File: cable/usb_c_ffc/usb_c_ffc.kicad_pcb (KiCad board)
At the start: 2 copper layers, 46.5 x 39.1 mm, 7 parts, among them J1 Conn_01x15_Socket, J2 Conn_01x15_Socket, J3 Conn_01x15_Socket, J4 Conn_01x15_Socket, J5 Conn_01x15_Socket, P1 TC-003LS, P2 TC-003LS

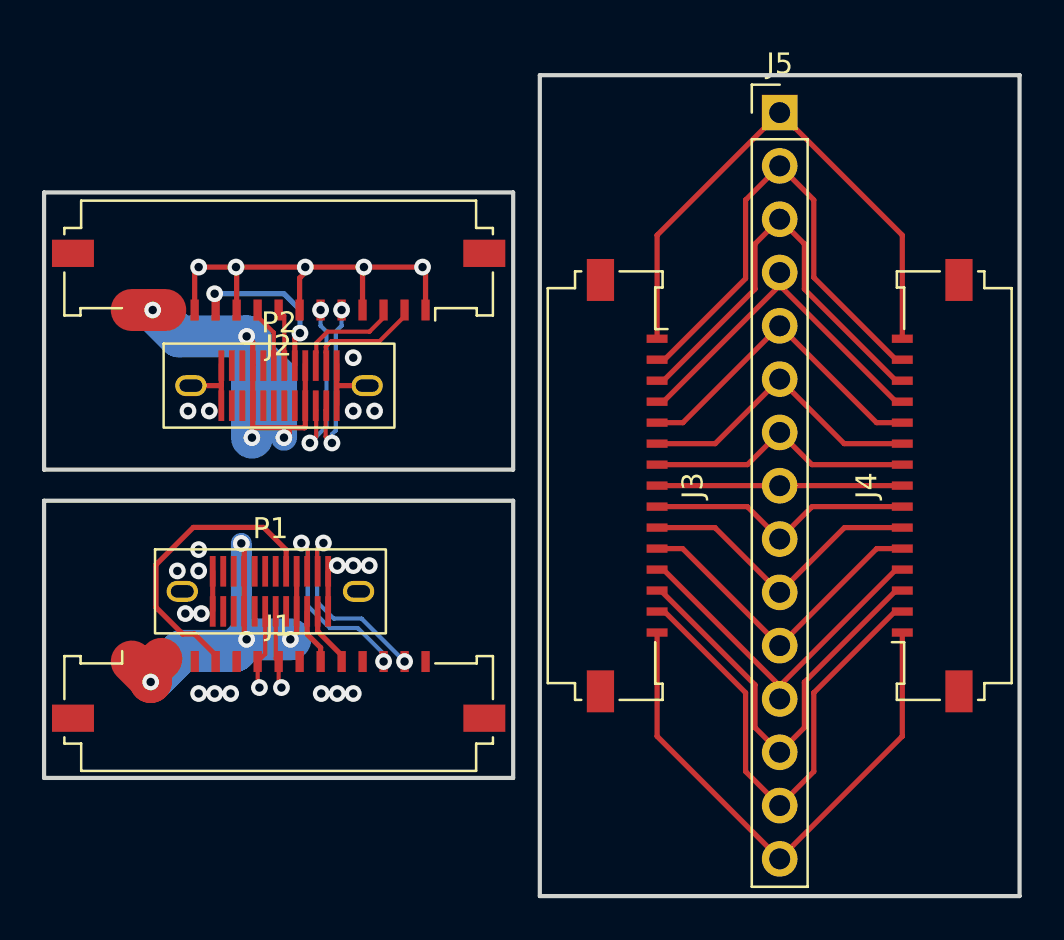
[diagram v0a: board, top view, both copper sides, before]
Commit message: cable pcb panel
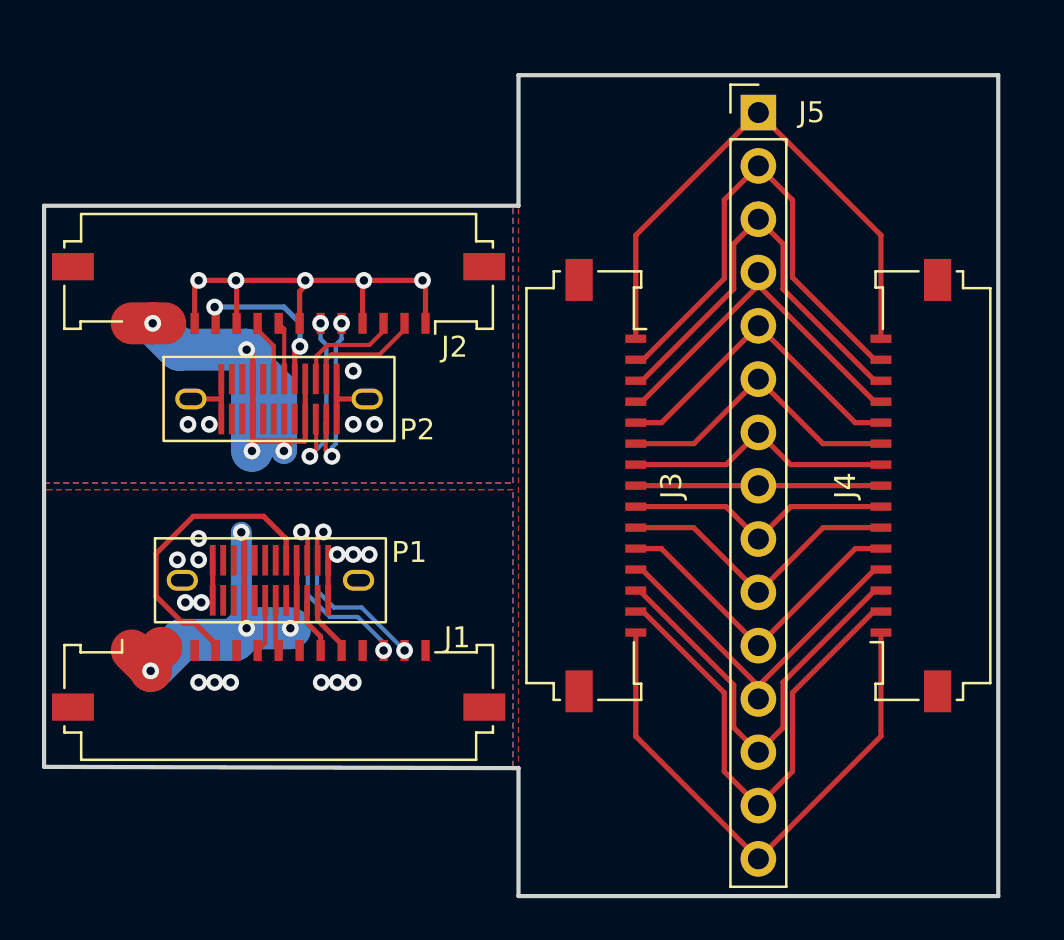
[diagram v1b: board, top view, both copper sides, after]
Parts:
- moved J3 1.02 mm to (64.6, 114.8)
- moved J5 1.02 mm to (71.4, 97.0)
- moved J4 1.02 mm to (78.1, 114.8)
- moved J2 0.64 mm to (48.5, 106.2)
- moved P2 0.63 mm to (48.5, 110.7)
- moved P1 0.53 mm to (48.1, 119.3)
- moved J1 0.53 mm to (48.5, 123.6)
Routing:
- net 1+: track 3.74 -> 2.45 mm, vias 1 -> 0
- net 1-: track 3.81 -> 2.54 mm, vias 1 -> 0
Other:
- board size 46.5 x 39.1 mm -> 45.5 x 39.1 mm
